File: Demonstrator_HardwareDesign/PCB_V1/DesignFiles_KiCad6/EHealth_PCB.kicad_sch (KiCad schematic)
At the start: 44 parts, among them J1 Conn_01x06, J2 Conn_01x06, J3-MagneticInterconnect1 Conn_01x08, J4 Conn_01x06, J4-OffTheShelf-Digital1 Conn_02x06_Counter_Clockwise, J5-Power1 Conn_01x03, J5-Power2 Conn_01x03, Q1 PMOS, U1 TCA9548APWR, U2 DEBO DCDC DOWN 4

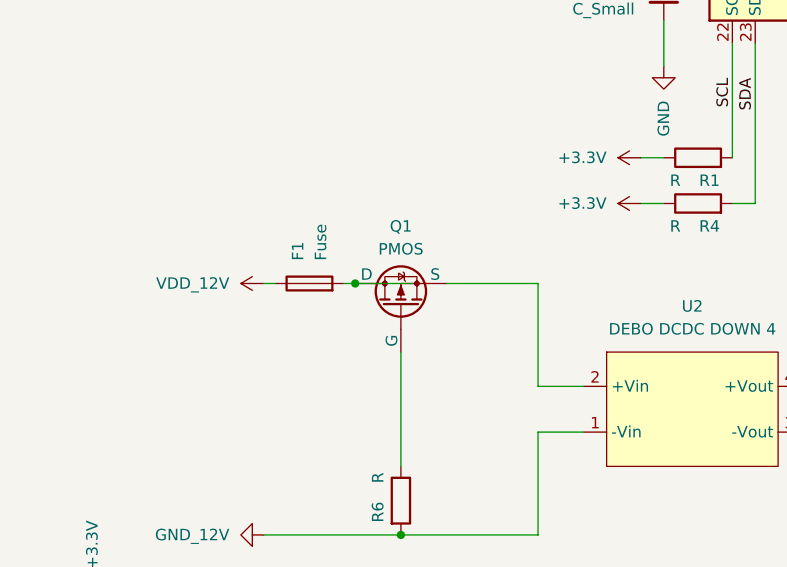
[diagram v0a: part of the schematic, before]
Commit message: up to date
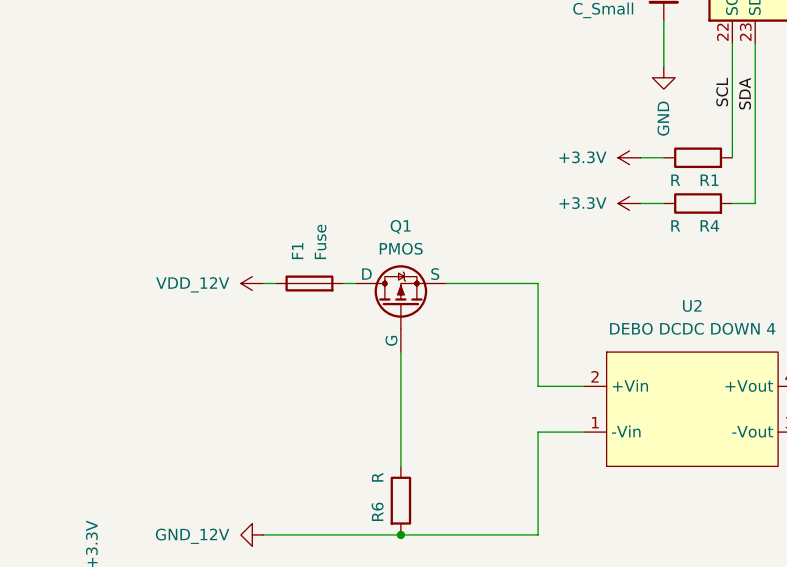
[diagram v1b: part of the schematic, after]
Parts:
- F1: footprint Fuse:Fuse_0402_1005Metric -> Fuse:Fuse_0805_2012Metric_Pad1.15x1.40mm_HandSolder
- Q1: footprint Package_TO_SOT_SMD:SOT-23_Handsoldering -> Package_SO:Infineon_PG-DSO-8-27_3.9x4.9mm_EP2.65x3mm
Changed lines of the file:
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@@
 	)
 	(junction
-		(at 68.58 132.08)
-		(diameter 0)
-		(color 0 0 0 0)
-	)
-	(junction
 		(at 161.29 26.67)
 		(diameter 0)
@@
 	(wire
 		(pts
-			(xy 74.93 132.08) (xy 68.58 132.08)
-		)
-		(stroke
-			(width 0)
-			(type default)
-		)
-	)
-	(wire
-		(pts
 			(xy 251.46 31.75) (xy 252.73 31.75)
 		)
@@
 			)
 		)
-		(property "Footprint" "Package_TO_SOT_SMD:SOT-23_Handsoldering"
+		(property "Footprint" "Package_SO:Infineon_PG-DSO-8-27_3.9x4.9mm_EP2.65x3mm"
 			(at 71.12 129.54 0)
 			(effects
@@
 			)
 		)
-		(property "Footprint" "Fuse:Fuse_0402_1005Metric"
+		(property "Footprint" "Fuse:Fuse_0805_2012Metric_Pad1.15x1.40mm_HandSolder"
 			(at 63.5 133.858 90)
 			(effects

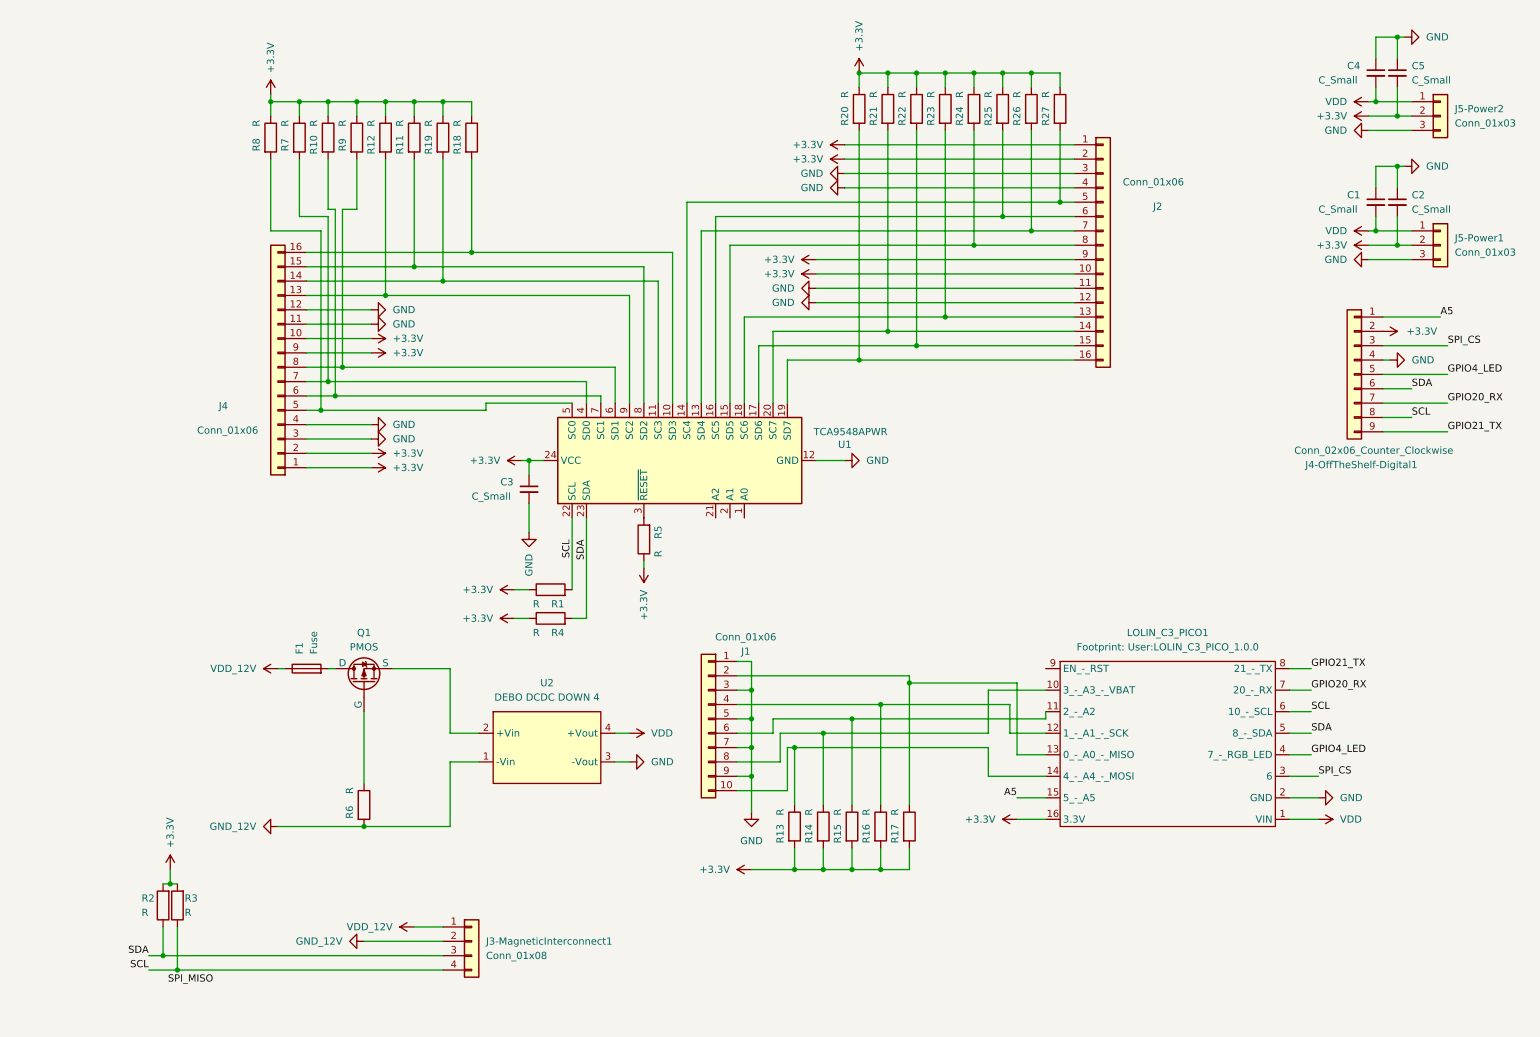
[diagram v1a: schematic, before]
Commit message: huidige layout
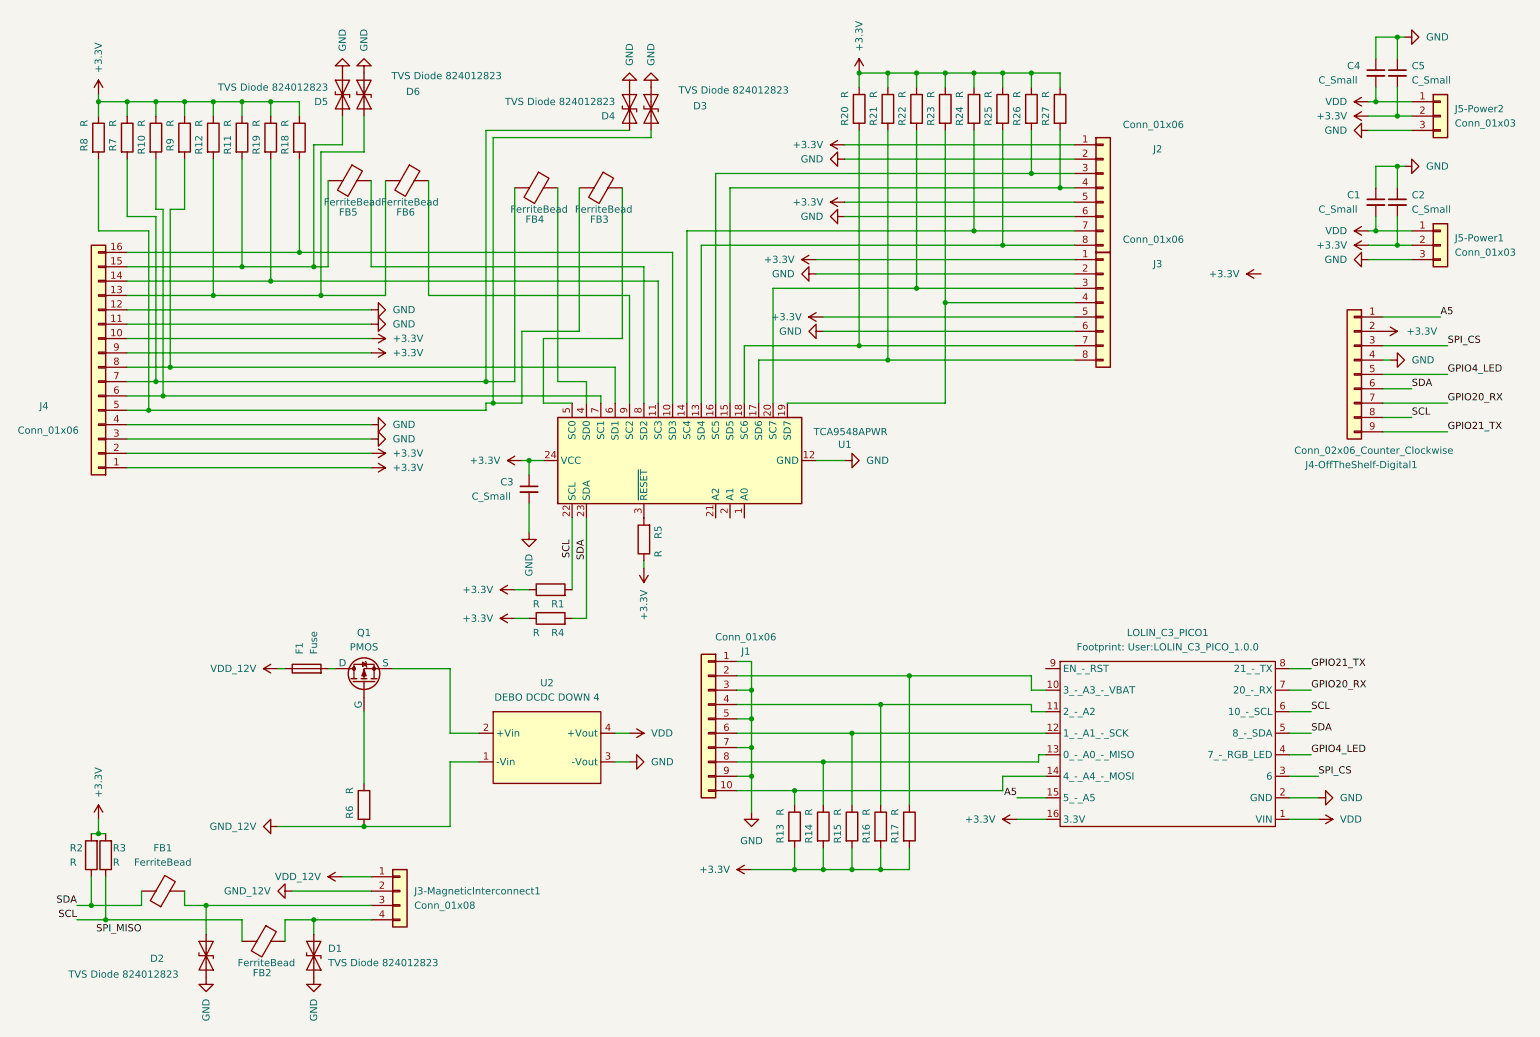
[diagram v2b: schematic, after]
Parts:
- removed J2: Conn_01x06, Connector_PinHeader_2.54mm:PinHeader_1x16_P2.54mm_Vertical, symbol Connector_Generic:Conn_01x16
- added D1, D4, D5: TVS Diode 824012823, Resistor_SMD:R_0603_1608Metric_Pad0.98x0.95mm_HandSolder, symbol Diode:SMAJ250CA
- added D2, D3, D6: TVS Diode 824012823, Resistor_SMD:R_0603_1608Metric_Pad0.98x0.95mm_HandSolder, symbol Diode:SMAJ400CA
- added FB1, FB2, FB3, FB4, FB5, FB6: FerriteBead, Resistor_SMD:R_0805_2012Metric_Pad1.20x1.40mm_HandSolder, symbol Device:FerriteBead
- added J2, J3: Conn_01x06, Connector_PinHeader_2.54mm:PinHeader_1x08_P2.54mm_Vertical, symbol Connector_Generic:Conn_01x08
- Q1: footprint Package_SO:Infineon_PG-DSO-8-27_3.9x4.9mm_EP2.65x3mm -> Library-TRANS:PG-TDSON-8
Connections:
- net +3.3V: now also J2.1 (Pin_1), J2.5 (Pin_5), J3.1 (Pin_1), J3.5 (Pin_5)
- net GND: now also D1.1 (A1), D2.1 (A1), D3.1 (A1), D4.1 (A1), D5.1 (A1), D6.1 (A1), J2.2 (Pin_2), J2.6 (Pin_6), J3.2 (Pin_2), J3.6 (Pin_6)
- net SCL: now also FB2.2; no longer J3-MagneticInterconnect1.4 (Pin_4)
- net SDA: now also FB1.1; no longer J3-MagneticInterconnect1.3 (Pin_3)
- net at J1.8 (Pin_8), R14.1: now also LOLIN_C3_PICO1.13 (0_-_A0_-_MISO); no longer LOLIN_C3_PICO1.10 (3_-_A3_-_VBAT)
- net at J1.6 (Pin_6), R15.1: now also LOLIN_C3_PICO1.12 (1_-_A1_-_SCK); no longer LOLIN_C3_PICO1.11 (2_-_A2)
- net at J1.4 (Pin_4), R16.1: now also LOLIN_C3_PICO1.11 (2_-_A2); no longer LOLIN_C3_PICO1.12 (1_-_A1_-_SCK)
- net at J1.2 (Pin_2), R17.1: now also LOLIN_C3_PICO1.10 (3_-_A3_-_VBAT); no longer LOLIN_C3_PICO1.13 (0_-_A0_-_MISO)
- net at U1.20 (SC7): now also R22.2, J3.3 (Pin_3); no longer R21.2
- net at R23.2: now also U1.19 (SD7), J3.4 (Pin_4); no longer U1.18 (SC6)
- net at U1.17 (SD6): now also R21.2, J3.8 (Pin_8); no longer R22.2
- net at R20.2: now also U1.18 (SC6), J3.7 (Pin_7); no longer U1.19 (SD7)
- net at U1.14 (SC4): now also R24.2, J2.7 (Pin_7); no longer R27.2
- net at U1.16 (SC5): now also R26.2, J2.3 (Pin_3); no longer R25.2
- net at U1.13 (SD4): now also R25.2, J2.8 (Pin_8); no longer R26.2
- net at U1.15 (SD5): now also R27.2, J2.4 (Pin_4); no longer R24.2
- net at J4.13 (Pin_13), R12.2: now also D6.2 (A2), FB6.2; no longer U1.9 (SC2)
- net at J4.15 (Pin_15), R11.2: now also D5.2 (A2), FB5.2; no longer U1.8 (SD2)
- net at J4.7 (Pin_7), R7.2: now also D4.2 (A2), FB4.2; no longer U1.4 (SD0)
- net at J4.5 (Pin_5), R8.2: now also D3.2 (A2), FB3.2; no longer U1.5 (SC0)
- new net: D2.2 (A2), FB1.2, J3-MagneticInterconnect1.3 (Pin_3)
- new net: D1.2 (A2), FB2.1, J3-MagneticInterconnect1.4 (Pin_4)
- new net: FB3.1, U1.5 (SC0)
- new net: FB4.1, U1.4 (SD0)
- new net: FB6.1, U1.9 (SC2)
- new net: FB5.1, U1.8 (SD2)
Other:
- moved on the sheet: J3-MagneticInterconnect1, J4, R10, R11, R12, R18, R19, R2, R3, R7, R8, R9
